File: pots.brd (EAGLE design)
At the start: 16.5 x 51.4 mm, 6 parts

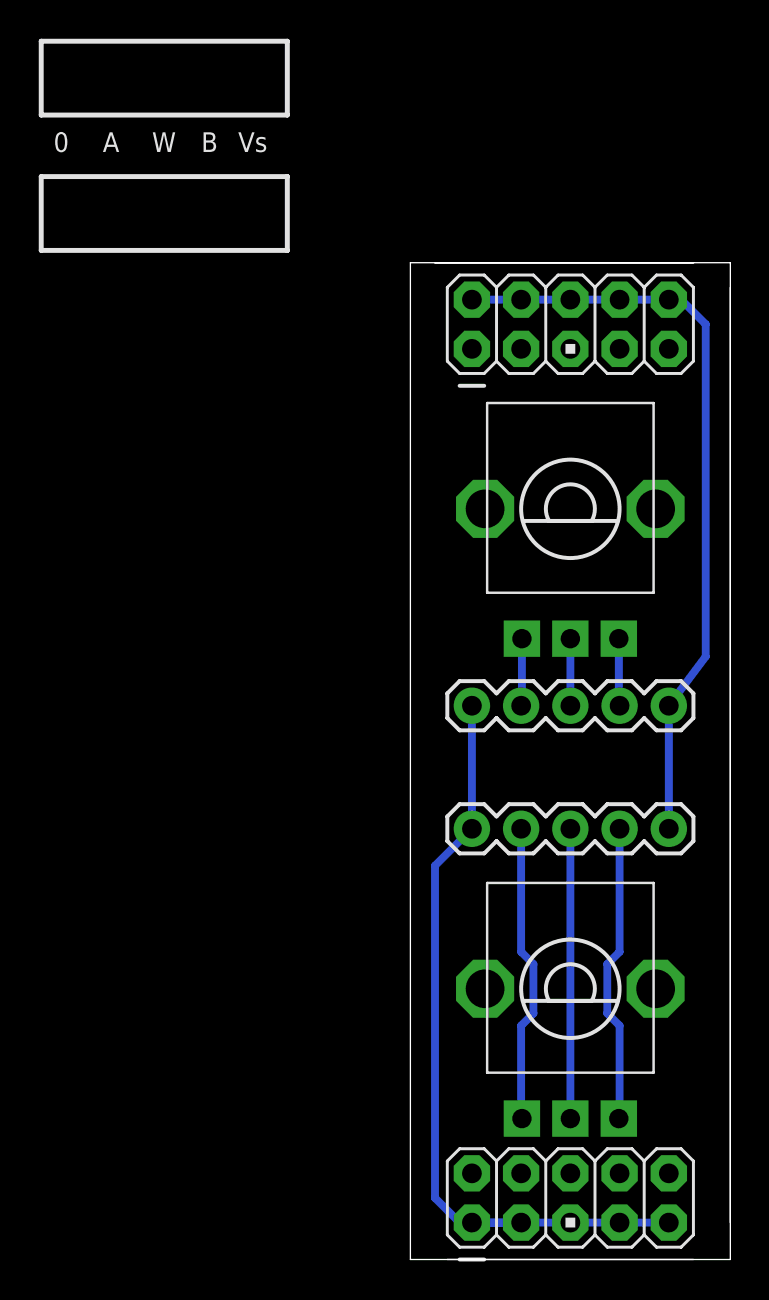
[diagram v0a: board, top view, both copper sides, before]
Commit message: Minor corrections
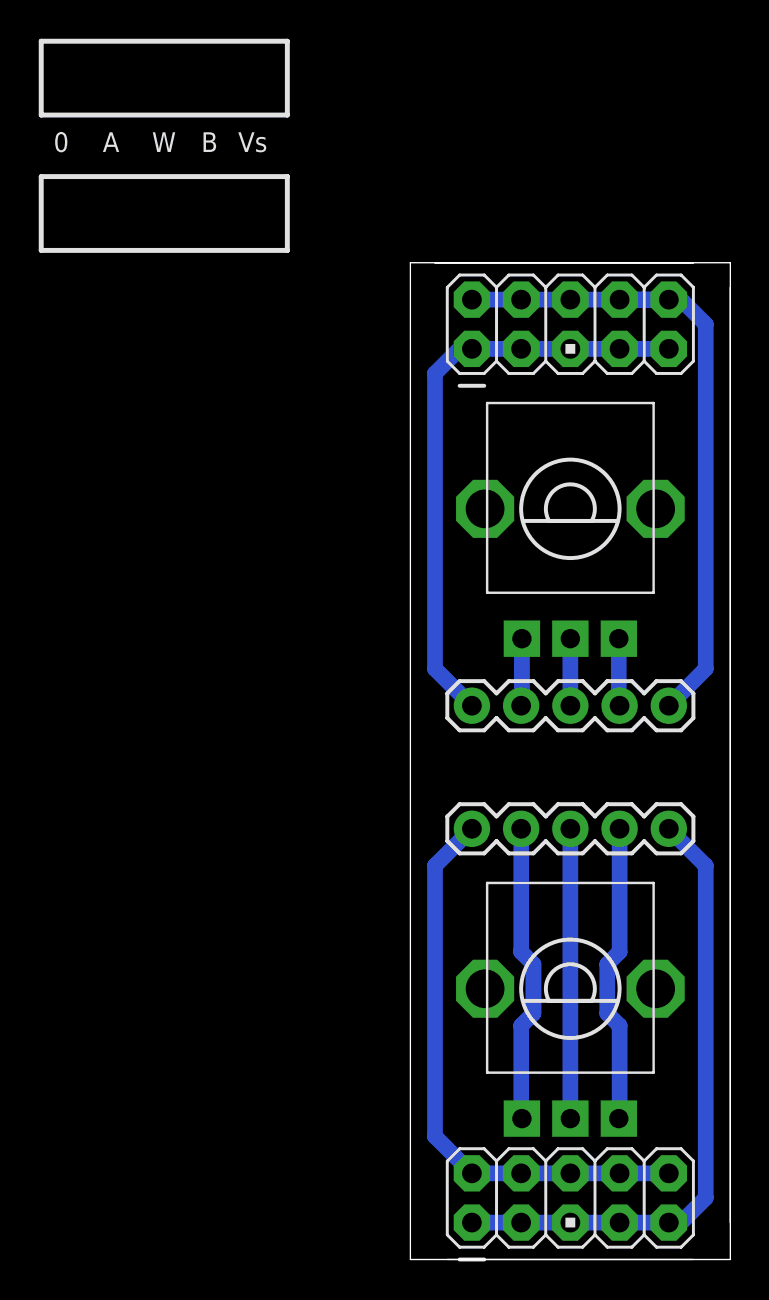
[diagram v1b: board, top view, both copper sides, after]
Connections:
- removed net VEE: JP2.1, JP2.3, JP2.5, JP2.7, JP2.9
- net VCC: now also JP2.1, JP2.3, JP2.5, JP2.7, JP2.9
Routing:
- net GND: track 0.00 -> 60.0 mm
- net VCC: track 39.3 -> 92.8 mm
- net VEE: track 42.0 -> 0.00 mm
- net N$4: track 3.46 -> 4.15 mm
- net N$2: track 3.46 -> 4.15 mm
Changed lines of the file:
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@@
 <contactref element="JP4" pad="1"/>
 <contactref element="JP3" pad="1"/>
+<wire x1="13.97" y1="47.625" x2="3.175" y2="47.625" width="0.8128" layer="16"/>
+<wire x1="3.175" y1="47.625" x2="1.905" y2="46.355" width="0.8128" layer="16"/>
+<wire x1="1.905" y1="46.355" x2="1.905" y2="31.115" width="0.8128" layer="16"/>
+<wire x1="1.905" y1="31.115" x2="3.81" y2="29.21" width="0.8128" layer="16"/>
+<wire x1="13.97" y1="5.08" x2="3.81" y2="5.08" width="0.8128" layer="16"/>
+<wire x1="3.81" y1="5.08" x2="1.905" y2="6.985" width="0.8128" layer="16"/>
+<wire x1="1.905" y1="6.985" x2="1.905" y2="20.955" width="0.8128" layer="16"/>
+<wire x1="1.905" y1="20.955" x2="3.81" y2="22.86" width="0.8128" layer="16"/>
+<wire x1="8.89" y1="47.625" x2="11.43" y2="47.625" width="0" layer="19" extent="1-1"/>
+<wire x1="6.35" y1="47.625" x2="8.89" y2="47.625" width="0" layer="19" extent="1-1"/>
+<wire x1="3.81" y1="47.625" x2="6.35" y2="47.625" width="0" layer="19" extent="1-1"/>
+<wire x1="3.175" y1="47.625" x2="3.81" y2="47.625" width="0" layer="19" extent="16-16"/>
+<wire x1="3.81" y1="22.86" x2="3.81" y2="29.21" width="0" layer="19" extent="1-1"/>
+<wire x1="11.43" y1="5.08" x2="13.97" y2="5.08" width="0" layer="19" extent="1-1"/>
+<wire x1="8.89" y1="5.08" x2="11.43" y2="5.08" width="0" layer="19" extent="1-1"/>
+<wire x1="6.35" y1="5.08" x2="3.81" y2="5.08" width="0" layer="19" extent="1-1"/>
 </signal>
 <signal name="VCC">
@@
 <contactref element="JP4" pad="5"/>
 <wire x1="3.81" y1="50.165" x2="8.89" y2="50.165" width="0.4064" layer="16"/>
-<wire x1="8.89" y1="50.165" x2="13.97" y2="50.165" width="0.4064" layer="16"/>
-<wire x1="13.97" y1="50.165" x2="14.605" y2="50.165" width="0.4064" layer="16"/>
-<wire x1="14.605" y1="50.165" x2="15.875" y2="48.895" width="0.4064" layer="16"/>
-<wire x1="13.97" y1="50.165" x2="11.43" y2="50.165" width="0" layer="19" extent="1-1"/>
-<wire x1="6.35" y1="50.165" x2="8.89" y2="50.165" width="0" layer="19" extent="1-1"/>
+<wire x1="8.89" y1="50.165" x2="11.43" y2="50.165" width="0.4064" layer="16"/>
 <wire x1="15.875" y1="48.895" x2="15.875" y2="31.75" width="0.4064" layer="16"/>
-<wire x1="15.875" y1="31.75" x2="13.97" y2="29.21" width="0.4064" layer="16"/>
-<wire x1="13.97" y1="22.86" x2="13.97" y2="29.21" width="0.4064" layer="16"/>
-</signal>
-<signal name="VEE">
 <contactref element="JP2" pad="7"/>
 <contactref element="JP2" pad="5"/>
@@
 <contactref element="JP2" pad="1"/>
 <contactref element="JP2" pad="9"/>
-<wire x1="13.97" y1="2.54" x2="6.35" y2="2.54" width="0.4064" layer="16"/>
-<wire x1="6.35" y1="2.54" x2="3.81" y2="2.54" width="0.4064" layer="16"/>
+<wire x1="13.97" y1="29.21" x2="15.875" y2="31.115" width="0.8128" layer="16"/>
+<wire x1="15.875" y1="31.115" x2="15.875" y2="48.895" width="0.8128" layer="16"/>
+<wire x1="11.43" y1="50.165" x2="13.97" y2="50.165" width="0.8128" layer="16"/>
+<wire x1="3.81" y1="50.165" x2="13.97" y2="50.165" width="0.8128" layer="16"/>
+<wire x1="13.97" y1="50.165" x2="14.605" y2="50.165" width="0.8128" layer="16"/>
+<wire x1="14.605" y1="50.165" x2="15.875" y2="48.895" width="0.8128" layer="16"/>
+<wire x1="3.81" y1="2.54" x2="13.97" y2="2.54" width="0.8128" layer="16"/>
+<wire x1="13.97" y1="2.54" x2="14.605" y2="2.54" width="0.8128" layer="16"/>
+<wire x1="14.605" y1="2.54" x2="15.875" y2="3.81" width="0.8128" layer="16"/>
+<wire x1="15.875" y1="3.81" x2="15.875" y2="20.955" width="0.8128" layer="16"/>
+<wire x1="15.875" y1="20.955" x2="13.97" y2="22.86" width="0.8128" layer="16"/>
+<wire x1="8.89" y1="50.165" x2="6.35" y2="50.165" width="0" layer="19" extent="1-1"/>
+<wire x1="13.97" y1="22.86" x2="13.97" y2="29.21" width="0" layer="19" extent="1-1"/>
+<wire x1="11.43" y1="2.54" x2="13.97" y2="2.54" width="0" layer="19" extent="1-1"/>
 <wire x1="8.89" y1="2.54" x2="11.43" y2="2.54" width="0" layer="19" extent="1-1"/>
-<wire x1="13.97" y1="2.54" x2="11.43" y2="2.54" width="0" layer="19" extent="1-1"/>
-<wire x1="6.35" y1="2.54" x2="3.175" y2="2.54" width="0.4064" layer="16"/>
-<wire x1="3.175" y1="2.54" x2="1.905" y2="3.81" width="0.4064" layer="16"/>
-<wire x1="1.905" y1="3.81" x2="1.905" y2="20.955" width="0.4064" layer="16"/>
-<wire x1="1.905" y1="20.955" x2="3.81" y2="22.86" width="0.4064" layer="16"/>
-<wire x1="3.81" y1="22.86" x2="3.81" y2="29.845" width="0.4064" layer="16"/>
-<wire x1="3.81" y1="29.845" x2="3.81" y2="2.54" width="0" layer="19" extent="1-16"/>
+<wire x1="6.35" y1="2.54" x2="3.81" y2="2.54" width="0" layer="19" extent="1-1"/>
 </signal>
 <signal name="N$2">
 <contactref element="JP3" pad="4"/>
 <contactref element="R23" pad="P$1"/>
-<wire x1="11.39" y1="32.67" x2="11.39" y2="29.885" width="0.4064" layer="16"/>
 <wire x1="11.39" y1="29.885" x2="11.43" y2="29.21" width="0.4064" layer="16"/>
+<wire x1="11.39" y1="32.67" x2="11.39" y2="29.25" width="0.8128" layer="16"/>
+<wire x1="11.39" y1="29.25" x2="11.43" y2="29.21" width="0.8128" layer="16"/>
 </signal>
 <signal name="N$3">
 <contactref element="JP3" pad="3"/>
 <contactref element="R23" pad="P$2"/>
-<wire x1="8.89" y1="32.67" x2="8.89" y2="29.21" width="0.4064" layer="16"/>
+<wire x1="8.89" y1="32.67" x2="8.89" y2="29.21" width="0.8128" layer="16"/>
 </signal>
 <signal name="N$4">
 <contactref element="JP3" pad="2"/>
 <contactref element="R23" pad="P$3"/>
-<wire x1="6.39" y1="32.67" x2="6.39" y2="29.885" width="0.4064" layer="16"/>
 <wire x1="6.39" y1="29.885" x2="6.35" y2="29.21" width="0.4064" layer="16"/>
+<wire x1="6.39" y1="32.67" x2="6.39" y2="29.25" width="0.8128" layer="16"/>
+<wire x1="6.39" y1="29.25" x2="6.35" y2="29.21" width="0.8128" layer="16"/>
 </signal>
 <signal name="N$5">
 <contactref element="JP4" pad="4"/>
 <contactref element="R1" pad="P$1"/>
-<wire x1="11.43" y1="22.86" x2="11.43" y2="16.51" width="0.4064" layer="16"/>
-<wire x1="11.43" y1="16.51" x2="10.795" y2="15.875" width="0.4064" layer="16"/>
-<wire x1="10.795" y1="15.875" x2="10.795" y2="13.335" width="0.4064" layer="16"/>
-<wire x1="10.795" y1="13.335" x2="11.43" y2="12.7" width="0.4064" layer="16"/>
-<wire x1="11.43" y1="12.7" x2="11.43" y2="7.945" width="0.4064" layer="16"/>
-<wire x1="11.43" y1="7.945" x2="11.39" y2="7.905" width="0.4064" layer="16"/>
+<wire x1="11.43" y1="12.7" x2="11.43" y2="7.945" width="0.8128" layer="16"/>
+<wire x1="11.43" y1="7.945" x2="11.39" y2="7.905" width="0.8128" layer="16"/>
+<wire x1="10.795" y1="15.875" x2="10.795" y2="13.335" width="0.8128" layer="16"/>
+<wire x1="10.795" y1="13.335" x2="11.43" y2="12.7" width="0.8128" layer="16"/>
+<wire x1="10.795" y1="15.875" x2="11.43" y2="16.51" width="0.8128" layer="16"/>
+<wire x1="11.43" y1="16.51" x2="11.43" y2="22.86" width="0.8128" layer="16"/>
 </signal>
 <signal name="N$6">
 <contactref element="JP4" pad="3"/>
 <contactref element="R1" pad="P$2"/>
-<wire x1="8.89" y1="22.86" x2="8.89" y2="7.905" width="0.4064" layer="16"/>
+<wire x1="8.89" y1="22.86" x2="8.89" y2="7.905" width="0.8128" layer="16"/>
 </signal>
 <signal name="N$7">
 <contactref element="JP4" pad="2"/>
 <contactref element="R1" pad="P$3"/>
-<wire x1="6.35" y1="22.86" x2="6.35" y2="16.51" width="0.4064" layer="16"/>
-<wire x1="6.35" y1="16.51" x2="6.985" y2="15.875" width="0.4064" layer="16"/>
-<wire x1="6.985" y1="15.875" x2="6.985" y2="13.335" width="0.4064" layer="16"/>
-<wire x1="6.985" y1="13.335" x2="6.35" y2="12.7" width="0.4064" layer="16"/>
-<wire x1="6.35" y1="12.7" x2="6.35" y2="7.945" width="0.4064" layer="16"/>
-<wire x1="6.35" y1="7.945" x2="6.39" y2="7.905" width="0.4064" layer="16"/>
+<wire x1="6.35" y1="22.86" x2="6.35" y2="16.51" width="0.8128" layer="16"/>
+<wire x1="6.35" y1="12.7" x2="6.35" y2="7.945" width="0.8128" layer="16"/>
+<wire x1="6.35" y1="7.945" x2="6.39" y2="7.905" width="0.8128" layer="16"/>
+<wire x1="6.985" y1="15.875" x2="6.985" y2="13.335" width="0.8128" layer="16"/>
+<wire x1="6.35" y1="12.7" x2="6.985" y2="13.335" width="0.8128" layer="16"/>
+<wire x1="6.985" y1="15.875" x2="6.35" y2="16.51" width="0.8128" layer="16"/>
 </signal>
 </signals>
